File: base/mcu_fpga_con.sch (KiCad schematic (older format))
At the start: 2 parts, among them J15 Conn_02x25_Odd_Even, J16 Conn_02x25_Odd_Even

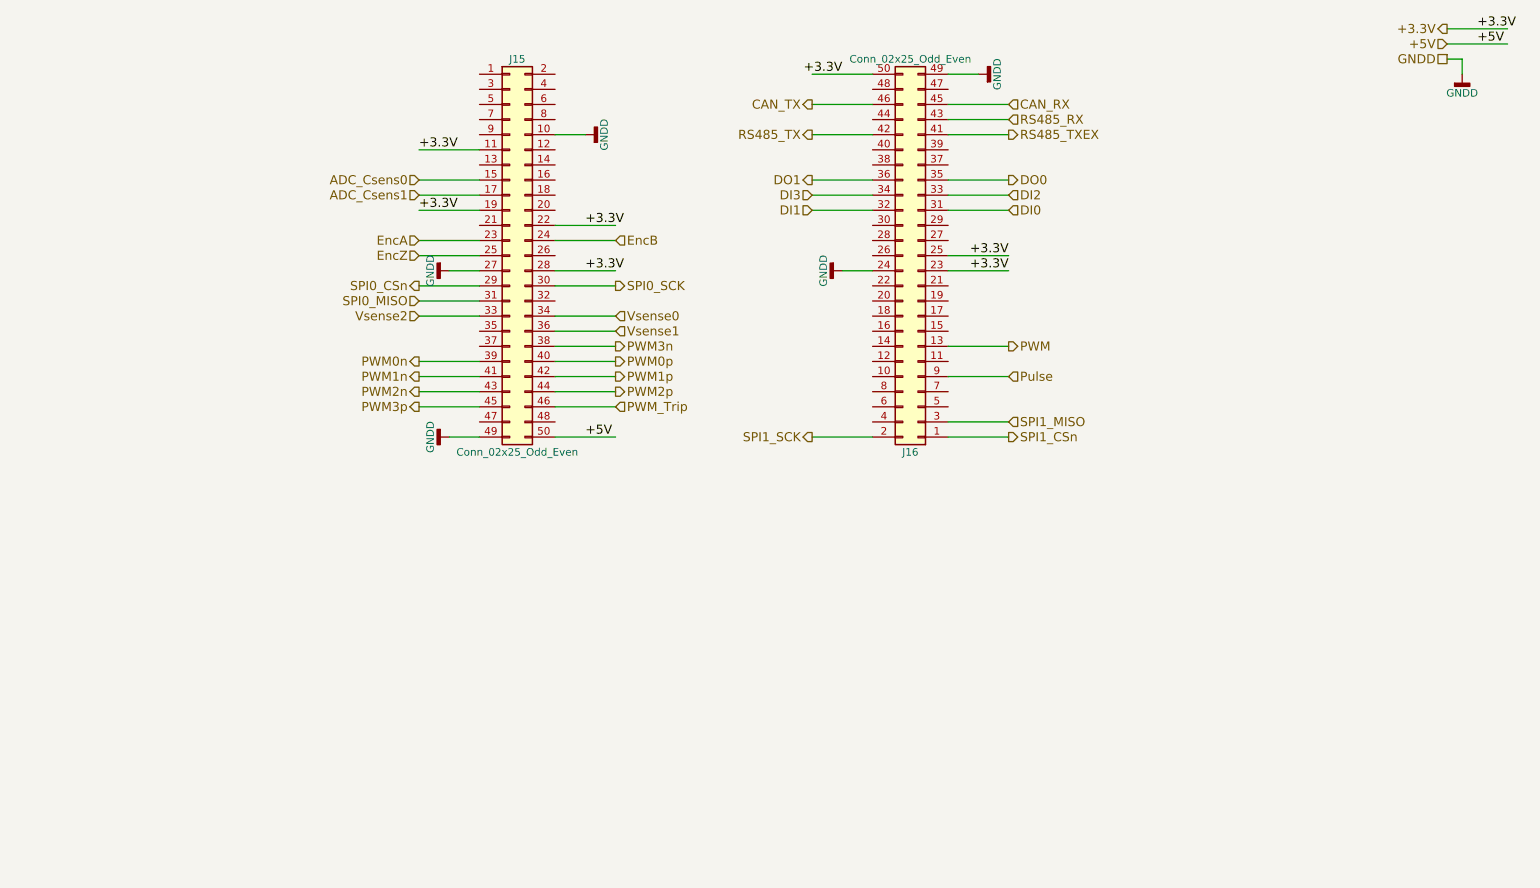
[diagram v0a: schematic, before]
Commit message: upd
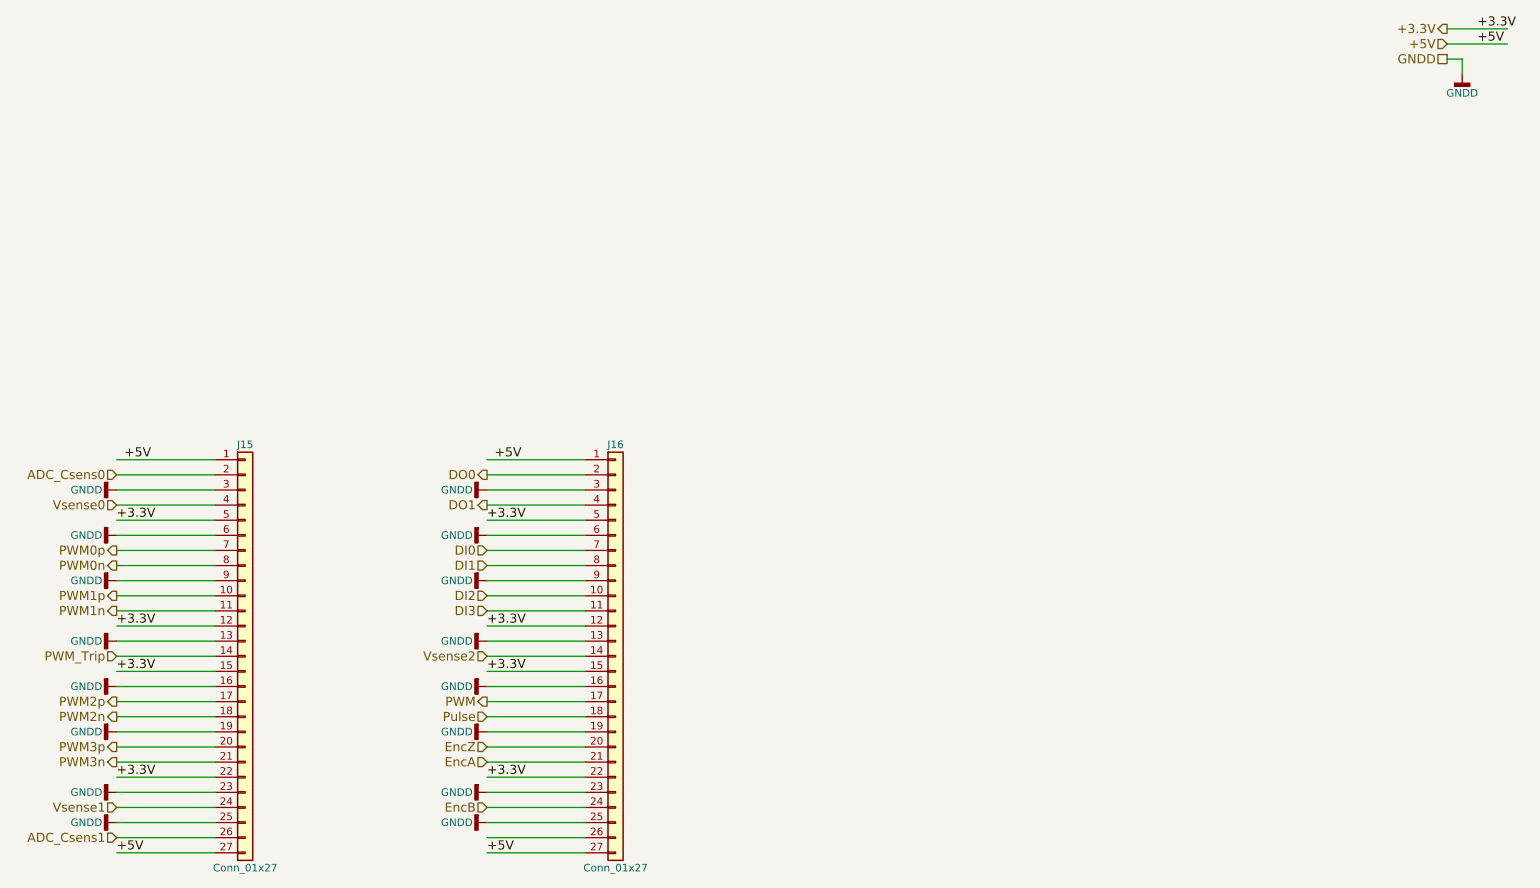
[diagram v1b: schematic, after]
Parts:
- removed J15, J16: Conn_02x25_Odd_Even, Connector_PinHeader_2.54mm:PinHeader_2x25_P2.54mm_Vertical, symbol Conn_02x25_Odd_Even
- added J15, J16: Conn_01x27, Connector_PinHeader_2.54mm:PinHeader_1x27_P2.54mm_Vertical, symbol Conn_01x27
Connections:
- net labels removed: CAN_RX, CAN_TX, RS485_RX, RS485_TX, RS485_TXEX, SPI0_CSn, SPI0_MISO, SPI0_SCK, SPI1_CSn, SPI1_MISO, SPI1_SCK
- wire segments 53 -> 58
